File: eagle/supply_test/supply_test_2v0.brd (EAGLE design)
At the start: 25.4 x 25.4 mm, 30 parts, among them J21 AC_INFILM, Q1 2N7002, U1 TPS62122

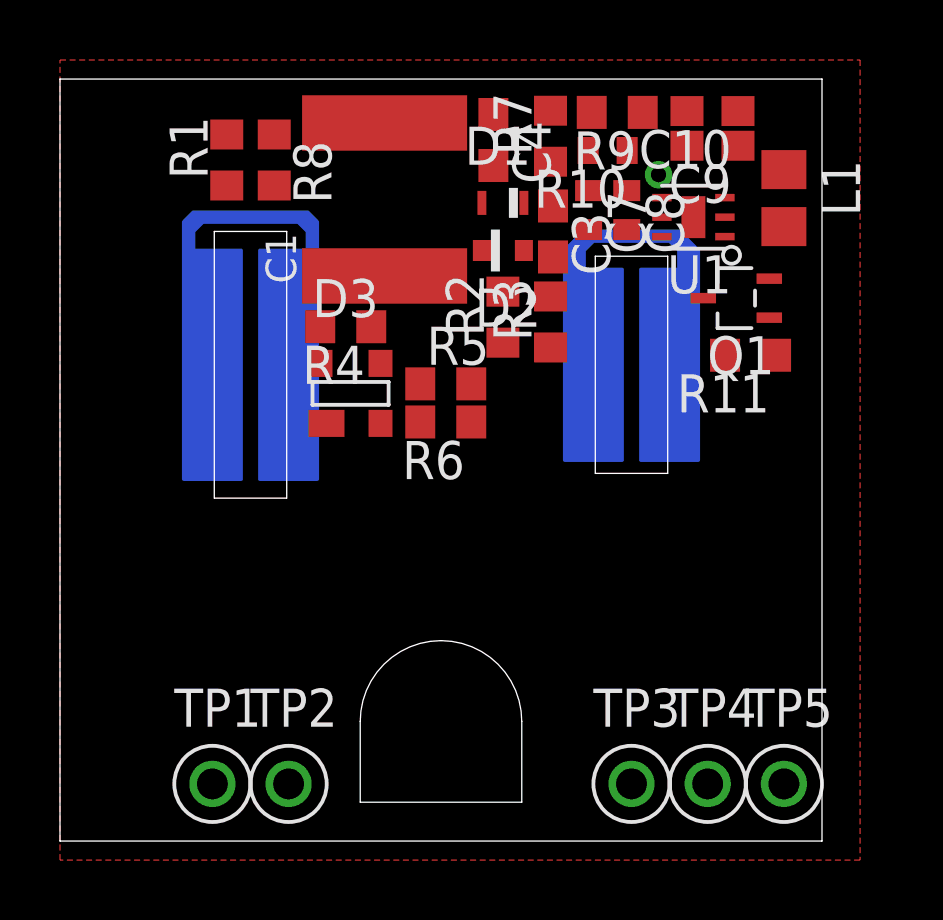
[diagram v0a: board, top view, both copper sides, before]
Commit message: routing
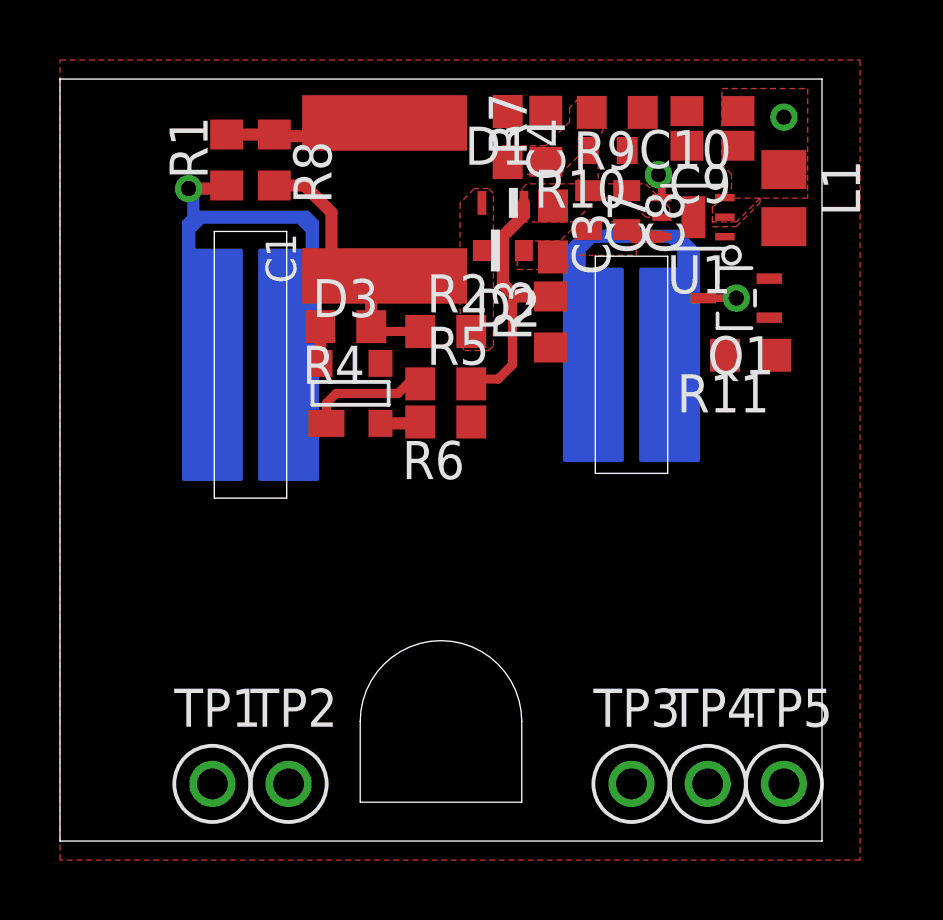
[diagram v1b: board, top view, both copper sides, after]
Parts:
- moved R2 1.96 mm to (0.16, 1.11), turned to 0 degrees
- moved C4 0.49 mm to (2.22, 7.59)
- moved R7 0.16 mm to (3.49, 7.62)
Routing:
- net N$4: track 0.00 -> 10.0 mm
- net VCC: track 0.00 -> 8.77 mm
- net N$2: track 0.00 -> 7.38 mm, vias 0 -> 1
- net N$1: track 0.00 -> 5.47 mm
- net N$7: track 0.00 -> 4.07 mm
- net N$16: track 0.00 -> 1.91 mm, vias 1 -> 2
- net N$8: track 0.00 -> 1.34 mm
- net GND: track 0.00 -> 1.27 mm
- net N$5: track 0.00 -> 1.23 mm
- added copper zone on layer 1, net +3V3
- added copper zone on layer 1, net N$13
- added copper zone on layer 1, net N$3
- added copper zone on layer 1, net VCC
